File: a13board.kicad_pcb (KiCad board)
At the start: 4 copper layers, 123.5 x 91.1 mm, 152 parts, among them P1 CONN_20, P2 CONN_20, P3 CONN_20, P4 CONN_20, P5 CONN_20, U1 H27UBG8T2A/TSOP48, U2 A13, U3 H5TQ2G43CFR, U4 H5TQ2G43CFR, U5 OLIMEX_IC_AXP209, U6 SY8008BAAC, U7 SY8008BAAC

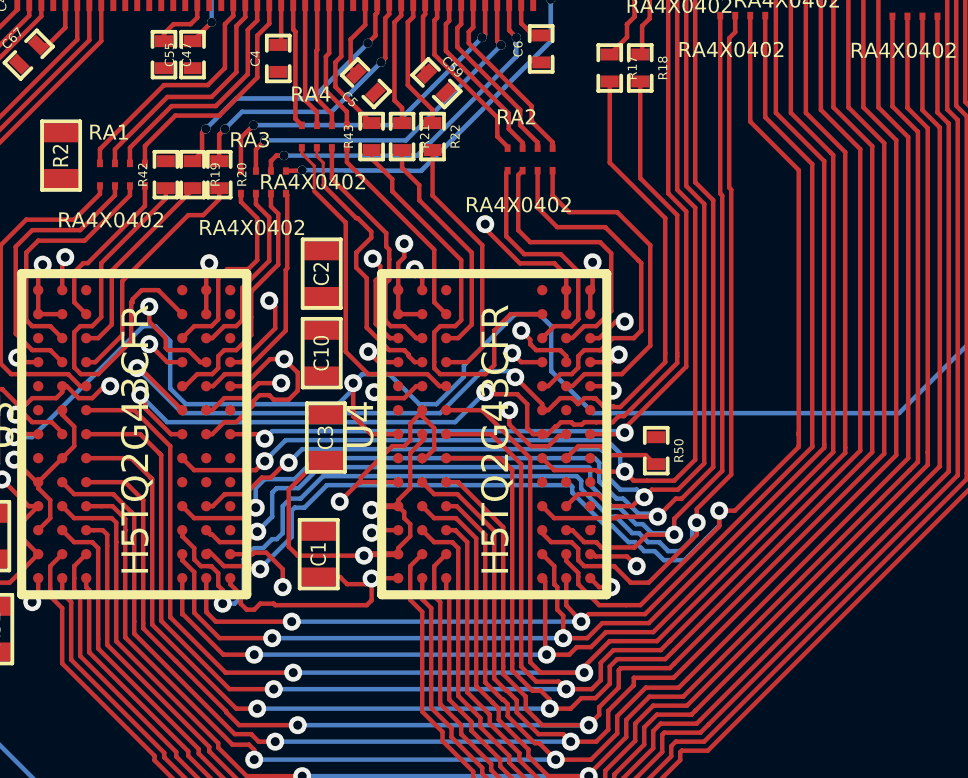
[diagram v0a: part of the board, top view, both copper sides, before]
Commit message: a bit improved layout
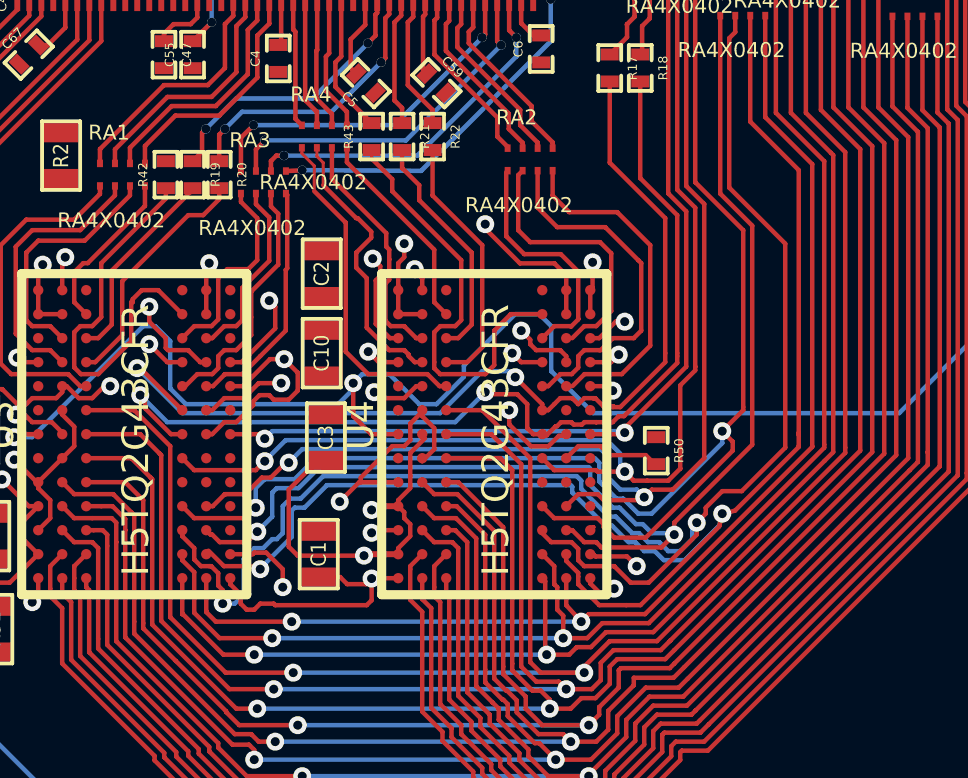
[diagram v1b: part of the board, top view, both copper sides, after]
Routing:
- net /DRAM/DDR3_A12: track 42.0 -> 47.2 mm
- net /DRAM/DDR3_A1: track 48.5 -> 50.4 mm
- net /DRAM/DDR3_A4: track 40.7 -> 41.6 mm
